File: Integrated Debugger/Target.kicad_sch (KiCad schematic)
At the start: 3 parts, among them J3 FPC socket 10P, J4 20021521-00010T1LF, SW1 RESET

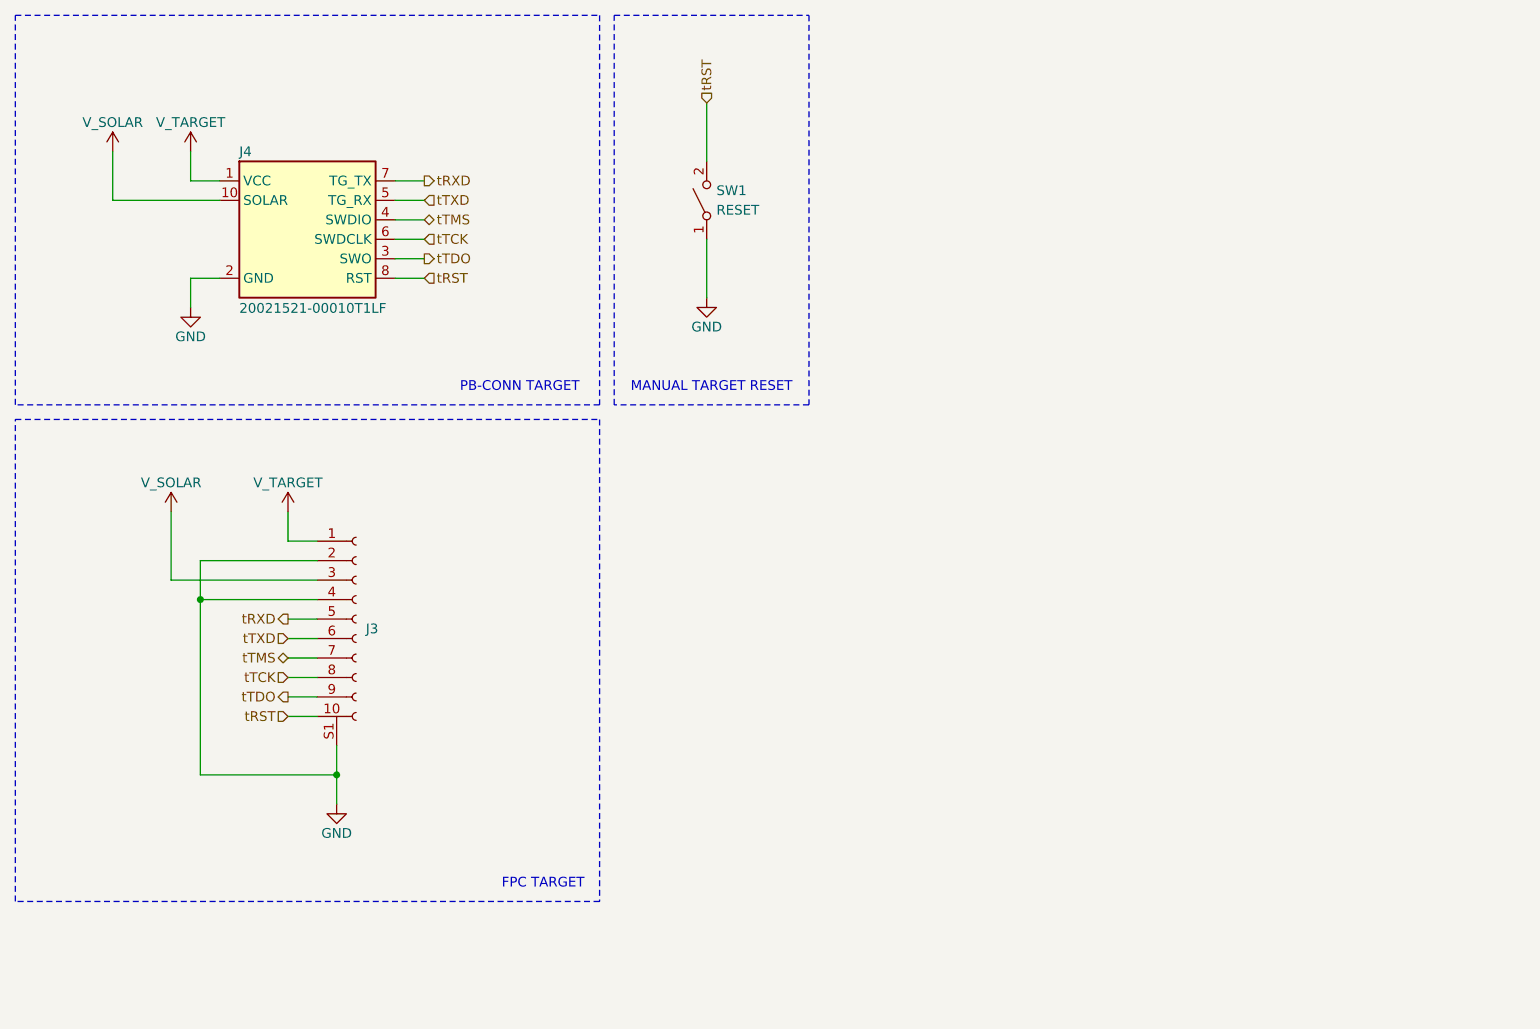
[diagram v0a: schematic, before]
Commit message: PCB improvements
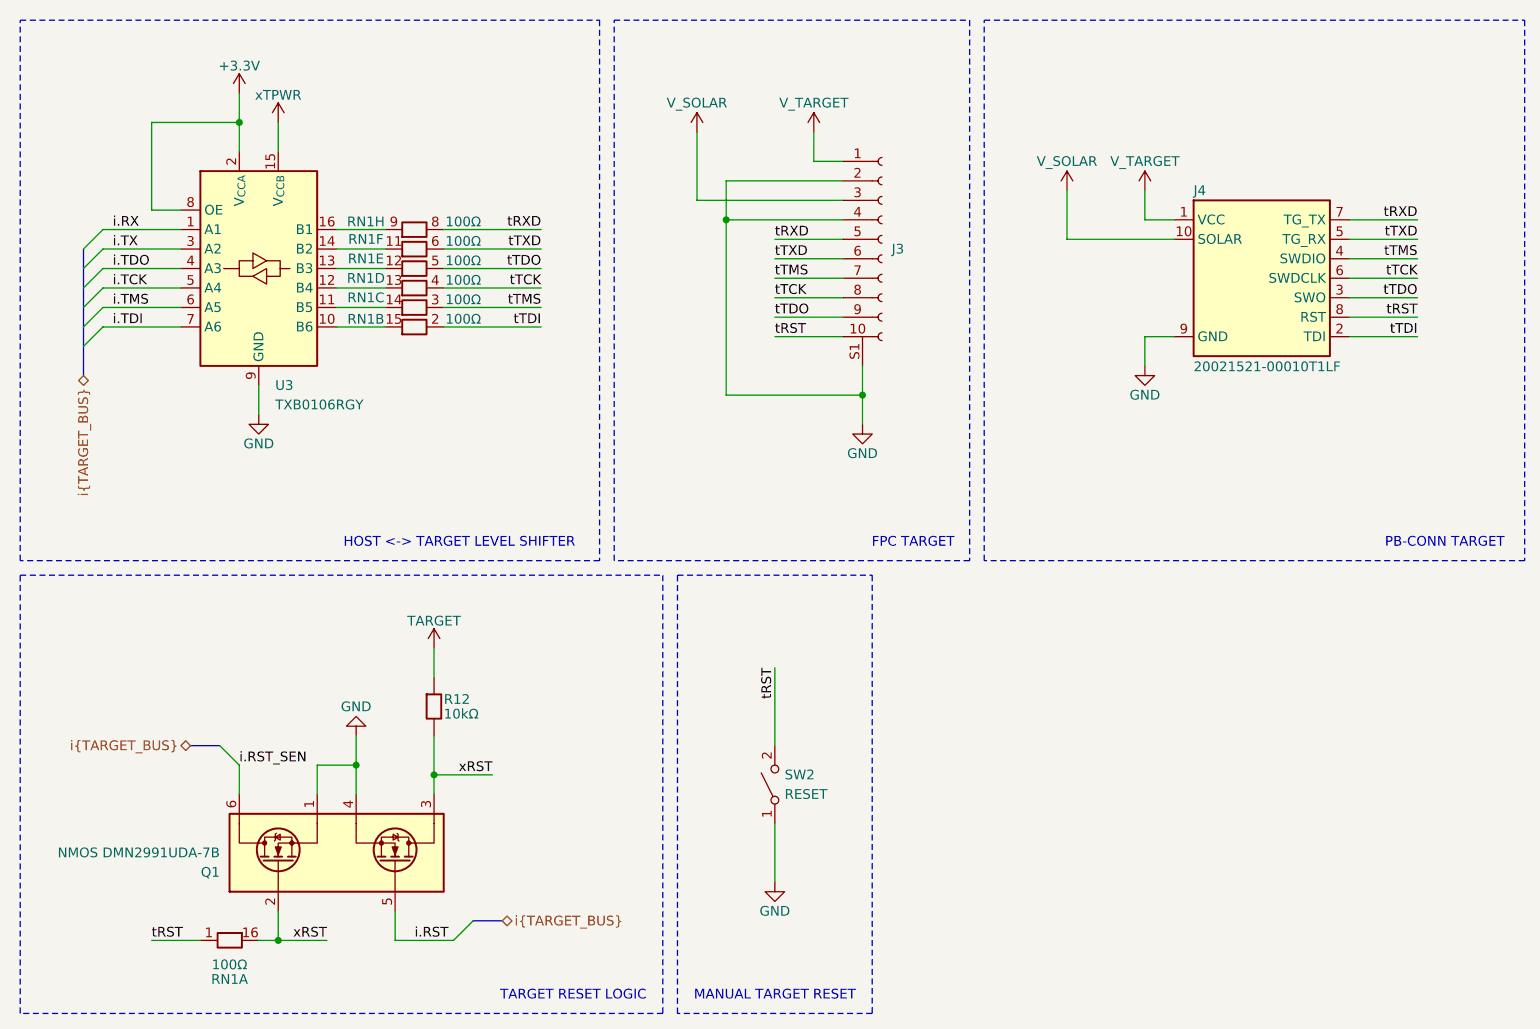
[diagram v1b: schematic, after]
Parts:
- added Q1: NMOS DMN2991UDA-7B, Picoballoon ICs:X2-DFN0806-6, symbol Picoballoon ICs:NMOS DMN2991UDA-7B
- added R12: 10kΩ, Picoballoon Passives:Resistor 0201, symbol Picoballoon Passives:Resistor
- added RN1: 100Ω, Picoballoon Passives:Resistor Pack YC248-JR-07100RL, symbol Picoballoon Passives:Resistor array 8
- added U3: TXB0106RGY, Picoballoon ICs:Texas_RGY_R-PVQFN-N16_EP2.05x2.55mm, symbol Picoballoon ICs:TXB0106RGY
- renumbered SW1 to SW2
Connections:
- net GND: now also Q1.1, Q1.4, U3.17 (GND), U3.9 (GND); no longer J4.2 (GND)
- net tRST: now also RN1.1 (R1.1)
- net tRXD: now also RN1.8 (R8.1)
- net tTCK: now also RN1.4 (R4.1)
- net tTDO: now also RN1.5 (R5.1)
- net tTMS: now also RN1.3 (R3.1)
- net tTXD: now also RN1.6 (R6.1)
- new net: RN1.15 (R2.2), U3.10 (B6)
- new net: RN1.13 (R4.2), U3.12 (B4)
- new net: RN1.12 (R5.2), U3.13 (B3)
- new net: RN1.9 (R8.2), U3.16 (B1)
- new net: RN1.14 (R3.2), U3.11 (B5)
- new net: RN1.11 (R6.2), U3.14 (B2)
- new net +3.3V: U3.2 (V_{CCA}), U3.8 (OE)
- new net TARGET: R12.1
- new net i.RST: Q1.5
- new net i.RST_SEN: Q1.6
- new net i.RX: U3.1 (A1)
- new net i.TCK: U3.5 (A4)
- new net i.TDI: U3.7 (A6)
- new net i.TDO: U3.4 (A3)
- new net i.TMS: U3.6 (A5)
- new net i.TX: U3.3 (A2)
- new net tTDI: J4.2 (TDI), RN1.2 (R2.1)
- new net xRST: Q1.2, Q1.3, R12.2, RN1.16 (R1.2)
- new net xTPWR: U3.15 (V_{CCB})
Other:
- note added: "HOST <-> TARGET LEVEL SHIFTER"
- note added: "TARGET RESET LOGIC"
- title: Target interface -> Target
- moved on the sheet: J3, SW2
